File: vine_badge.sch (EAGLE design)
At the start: 46 parts

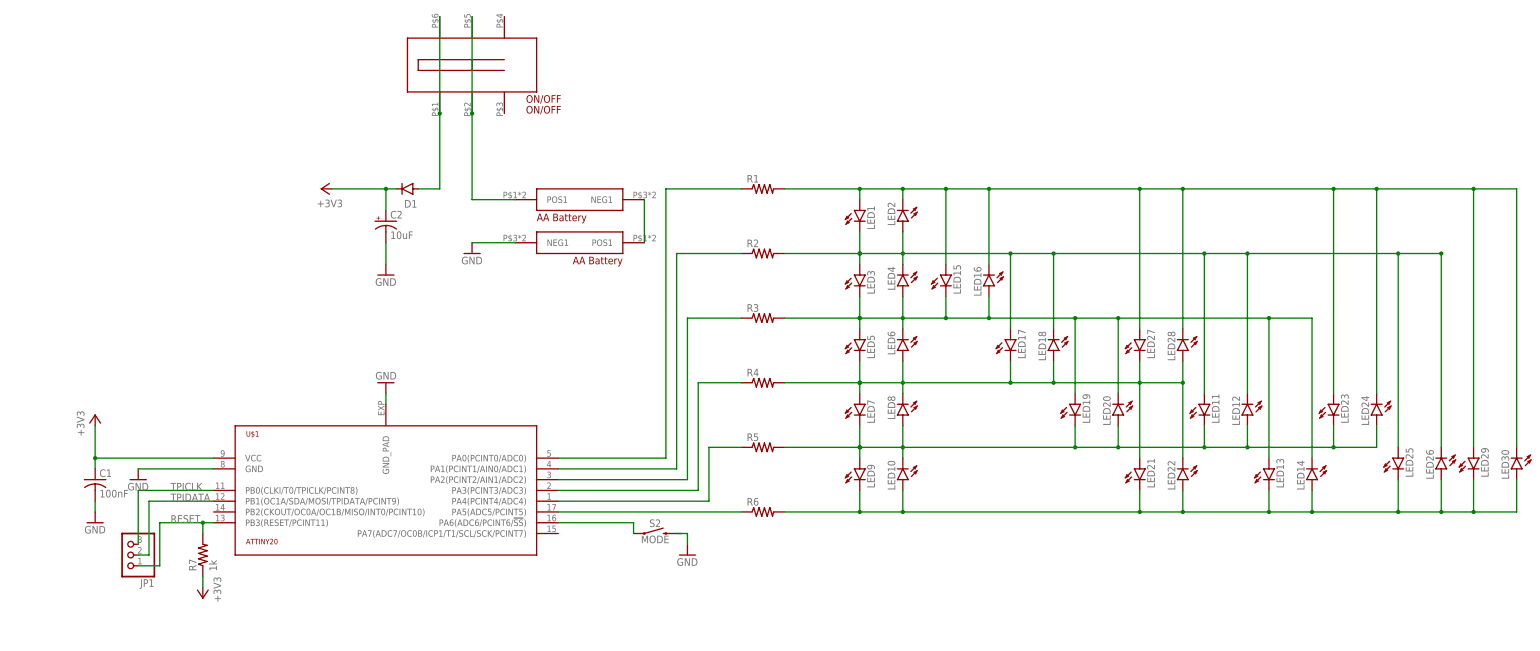
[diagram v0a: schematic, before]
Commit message: moved to v 1.1
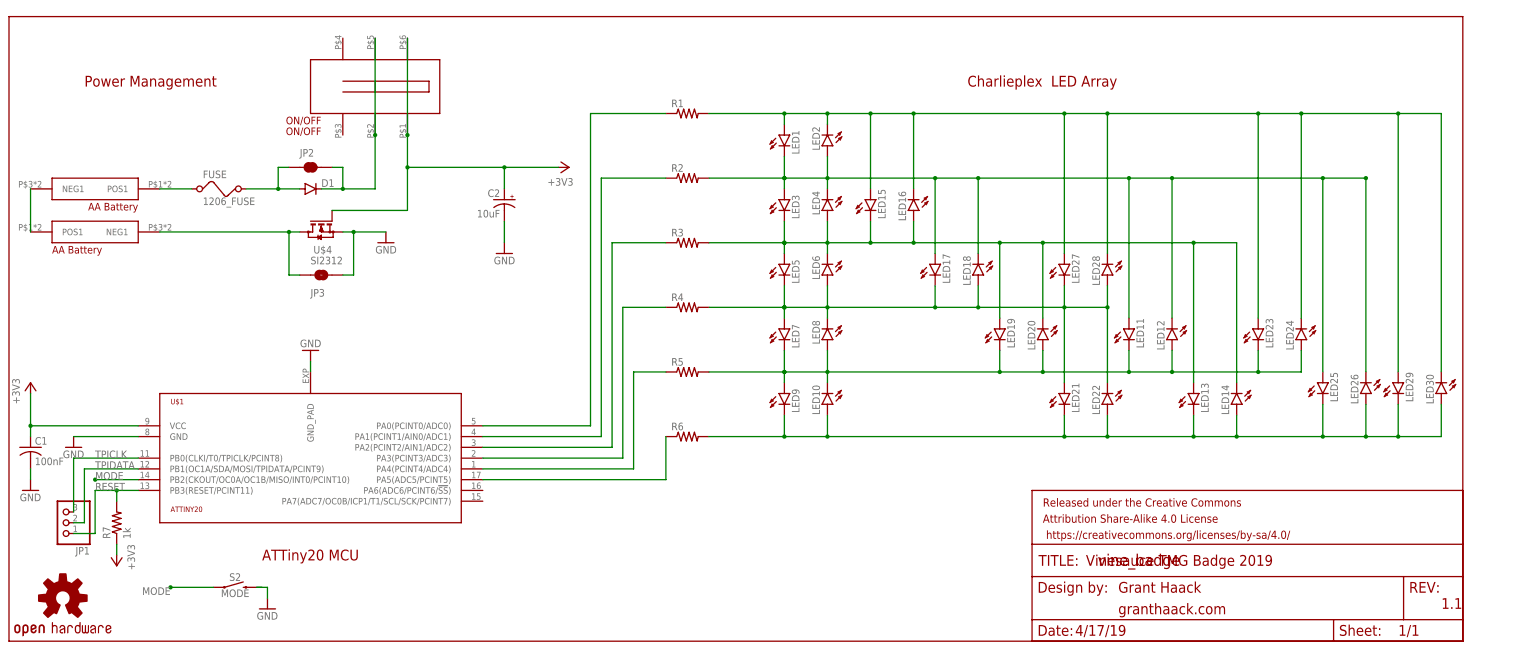
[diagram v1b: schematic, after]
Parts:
- added FRAME1: FRAME-LETTER, SparkFun-Aesthetics:FRAME-LETTER
- added FUSE: 1206_FUSE, VineBadge:1206_FUSE
- added JP2: JUMPER-SMT_2_NC_TRACE_NO-SILK, SparkFun-Jumpers:JUMPER-SMT_2_NC_TRACE_NO-SILK
- added JP3: JUMPER-SMT_2_NO_NO-SILK, SparkFun-Jumpers:JUMPER-SMT_2_NO_NO-SILK
- added LOGO1: OSHW-LOGOS-COPPER, SparkFun-Aesthetics:OSHW-LOGOS-COPPER
- added U$4: SI2312, VineBadge:SI2312
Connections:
- new net MODE: S2.1, U$1G$2.PB2(CKOUT/OC0A/OC1B/MISO/INT0/PCINT10)
- new net N$23: D1.C, JP2.2, ON/OFF.P$2, ON/OFF.P$5
- net +3V3: now also ON/OFF.P$1, ON/OFF.P$6, U$4.G; no longer D1.C
- net GND: now also JP3.2, U$4.S; no longer U$3.NEG1
- net N$18: now also FUSE.1, U$2.POS1; no longer S2.1, U$1G$2.PA6(ADC6/PCINT6/!SS!)
- net N$19: now also JP3.1, U$3.NEG1, U$4.D; no longer ON/OFF.P$2, ON/OFF.P$5, U$2.POS1
- net N$20: now also FUSE.2, JP2.1; no longer ON/OFF.P$1, ON/OFF.P$6
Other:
- note added: "1.1"
- note added: "4/17/19"
- note added: "ATTiny20 MCU"
- note added: "Charlieplex LED Array"
- note added: "Grant Haack"
- note added: "Power Management"
- note added: "Vinesauce TMG Badge 2019"
- note added: "granthaack.com"
- moved on the sheet: C1, C2, D1, JP1, LED1, LED10, LED11, LED12, LED13, LED14, LED15, LED16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
